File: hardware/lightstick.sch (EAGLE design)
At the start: 14 parts, among them U1 MCP1703AT-3302E/CB

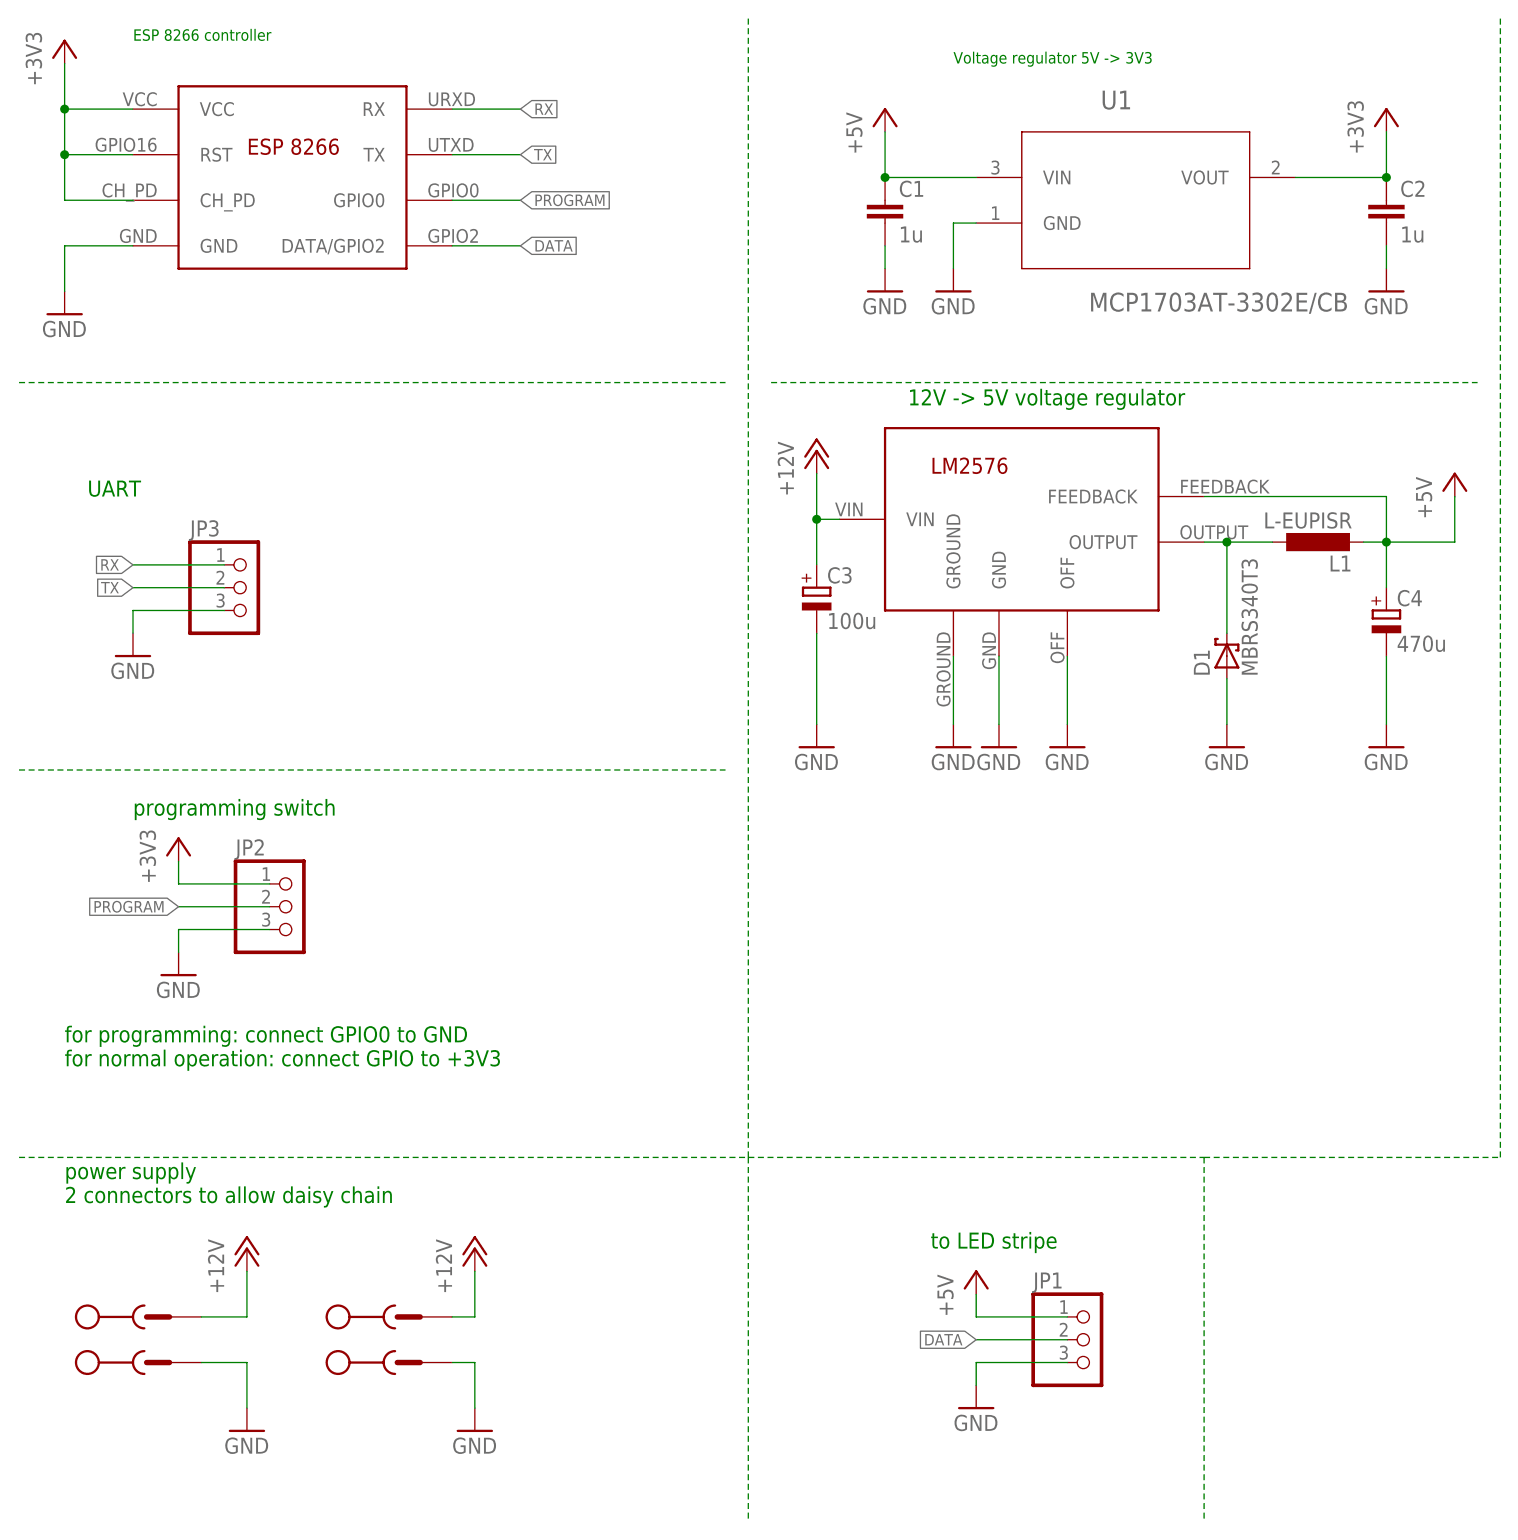
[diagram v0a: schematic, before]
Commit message: rerouting to accomodate easier soldering. connected GND top and bottom planes
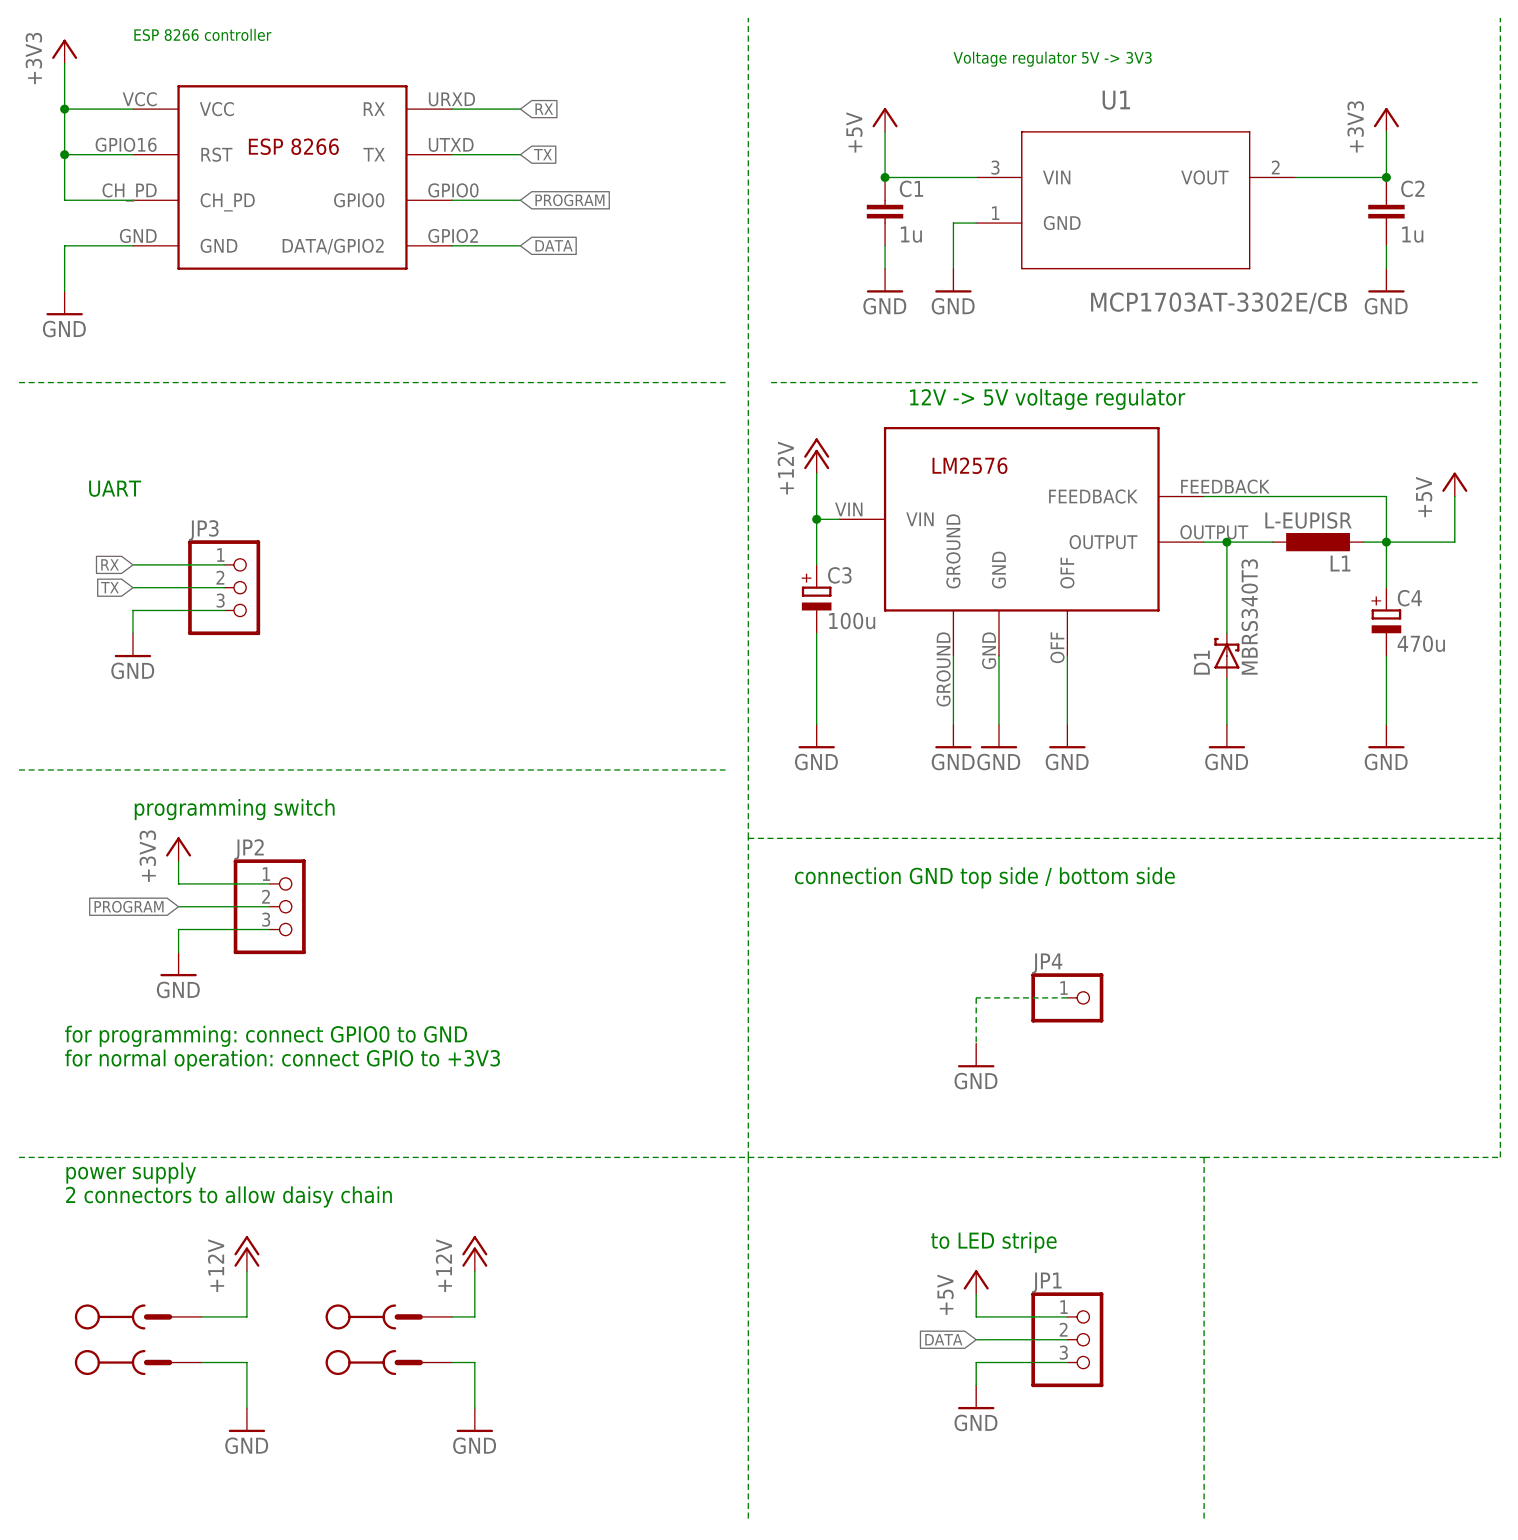
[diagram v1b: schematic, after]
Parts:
- added JP4: (no value), pinhead:PINHD-1X1
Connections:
- net GND: now also JP4.1
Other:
- note added: "connection GND top side / bottom side"
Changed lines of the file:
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@@
 <part name="U$3" library="lightstick" deviceset="AKL383-02" device=""/>
 <part name="U$4" library="lightstick" deviceset="AKL383-02" device=""/>
+<part name="JP4" library="pinhead" deviceset="PINHD-1X1" device=""/>
+<part name="GND16" library="supply1" deviceset="GND" device=""/>
 </parts>
 <sheets>
@@
 <text x="17.78" y="170.18" size="1.27" layer="91">ESP 8266 controller</text>
 <text x="104.14" y="129.54" size="1.778" layer="91">12V -&gt; 5V voltage regulator</text>
+<text x="91.44" y="76.2" size="1.778" layer="91">connection GND top side / bottom side</text>
 </plain>
 <instances>
@@
 <instance part="U$3" gate="G$1" x="40.64" y="22.86"/>
 <instance part="U$4" gate="G$1" x="12.7" y="22.86"/>
+<instance part="JP4" gate="G$1" x="124.46" y="63.5"/>
+<instance part="GND16" gate="1" x="111.76" y="55.88"/>
 </instances>
 <busses>
@@
 <wire x1="30.48" y1="17.78" x2="30.48" y2="22.86" width="0.1524" layer="91"/>
 <wire x1="30.48" y1="22.86" x2="25.4" y2="22.86" width="0.1524" layer="91"/>
+</segment>
+<segment>
+<pinref part="JP4" gate="G$1" pin="1"/>
+<pinref part="GND16" gate="1" pin="GND"/>
+<wire x1="121.92" y1="63.5" x2="111.76" y2="63.5" width="0.1524" layer="91" style="longdash"/>
+<wire x1="111.76" y1="63.5" x2="111.76" y2="58.42" width="0.1524" layer="91" style="longdash"/>
 </segment>
 </net>
@@
 <wire x1="137.16" y1="45.72" x2="137.16" y2="5.08" width="0.1524" layer="91" style="longdash"/>
 <wire x1="86.36" y1="45.72" x2="86.36" y2="5.08" width="0.1524" layer="91" style="longdash"/>
-<wire x1="86.36" y1="45.72" x2="86.36" y2="172.72" width="0.1524" layer="91" style="longdash"/>
-<wire x1="170.18" y1="45.72" x2="170.18" y2="172.72" width="0.1524" layer="91" style="longdash"/>
+<wire x1="86.36" y1="45.72" x2="86.36" y2="81.28" width="0.1524" layer="91" style="longdash"/>
+<wire x1="86.36" y1="81.28" x2="86.36" y2="172.72" width="0.1524" layer="91" style="longdash"/>
+<wire x1="170.18" y1="45.72" x2="170.18" y2="81.28" width="0.1524" layer="91" style="longdash"/>
+<wire x1="170.18" y1="81.28" x2="170.18" y2="172.72" width="0.1524" layer="91" style="longdash"/>
 <wire x1="137.16" y1="45.72" x2="170.18" y2="45.72" width="0.1524" layer="91" style="longdash"/>
+<wire x1="86.36" y1="81.28" x2="170.18" y2="81.28" width="0.1524" layer="91" style="longdash"/>
 </segment>
 </net>
@@
 </sheet>
 </sheets>
+<errors>
+</errors>
 </schematic>
 </drawing>
